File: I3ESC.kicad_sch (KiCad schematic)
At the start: 120 parts, among them J1 JST SR/SZ, J10 VIN_BARREL, J11 Barrel_Jack, J12 JST SR/SZ, J13 Conn_01x04, J2 Screw_Terminal_01x02, J3 Screw_Terminal_01x02, J4 Screw_Terminal_01x02, J5 Conn_01x06, J6 Wireless Coil, J7 VIN_TERMINAL, J8 Conn_01x06, J9 JST SR/SZ, SW2 boot-red, SW3 user1-white, U1 SY8113BADC, U10 USBLC6-2P6, U11 IP6826, U12 FD8288T (DRV8300), U2 FD8288T (DRV8300), U3 SPX3819M5-L-3-3, U4 STM32G474RETx, U5 Qwiic1, U6 USB_C_Receptacle, U8 ABM3B-8.000MHZ, U9 USB_C_Receptacle

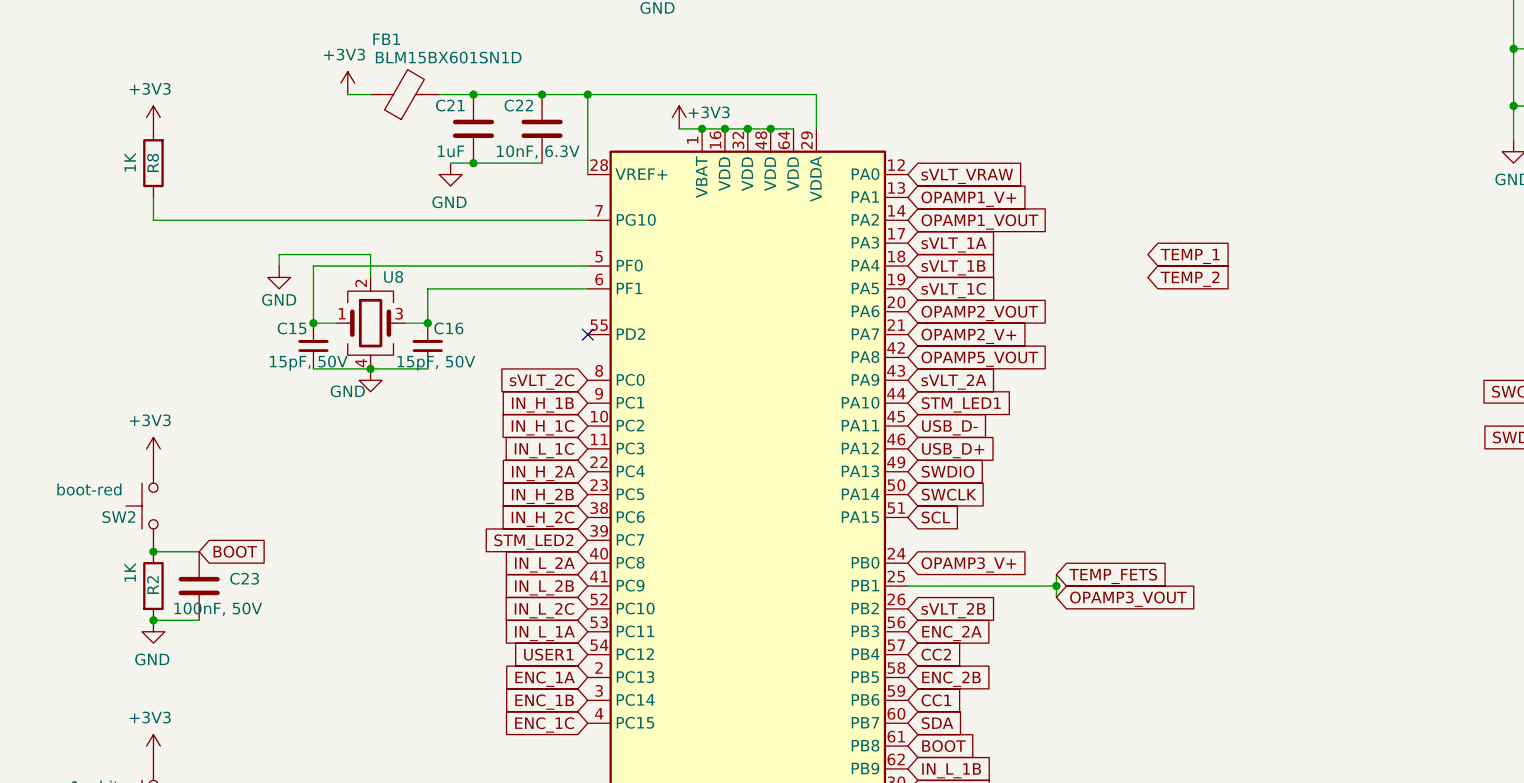
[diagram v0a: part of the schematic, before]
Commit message: majority of routing for V2 completed
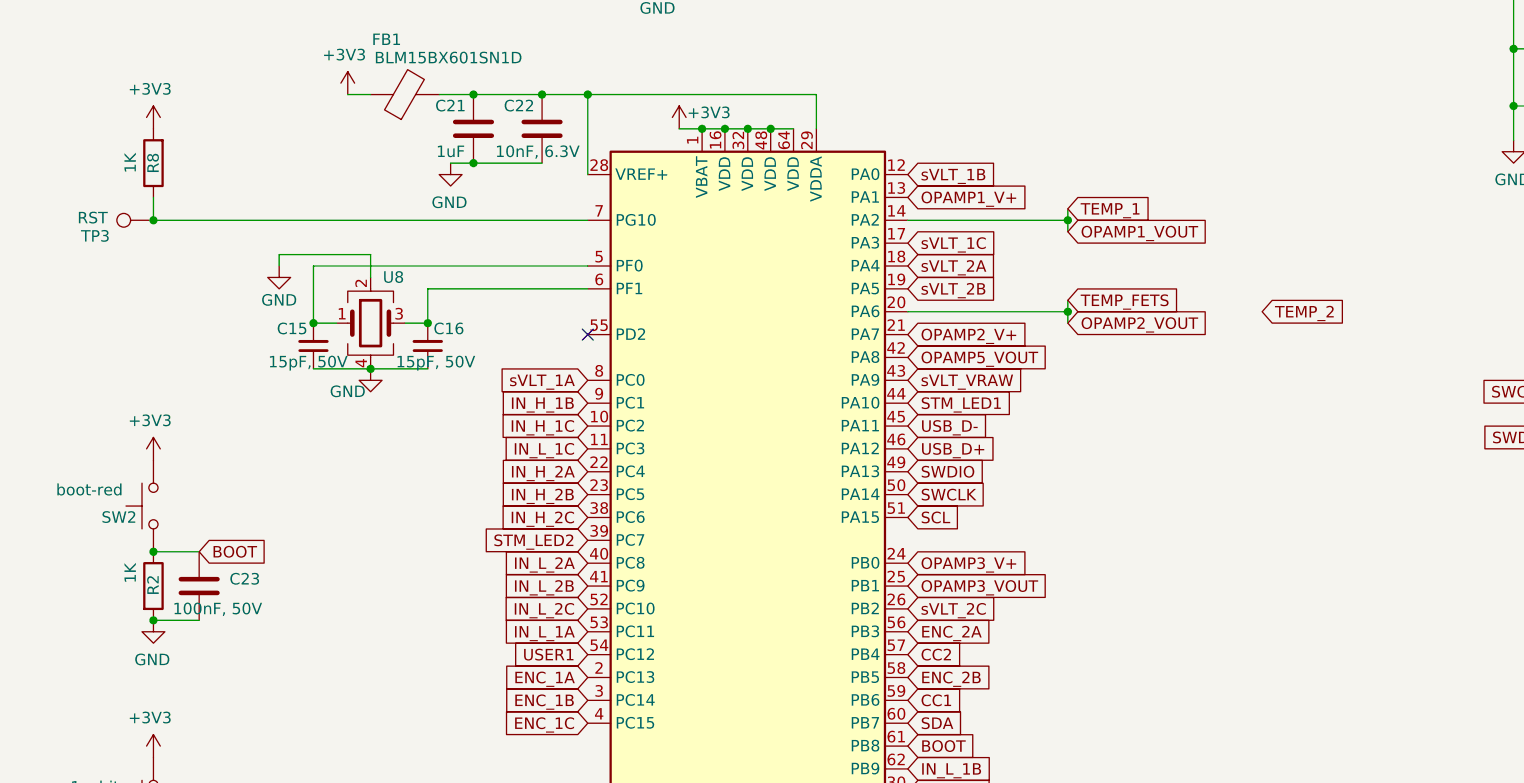
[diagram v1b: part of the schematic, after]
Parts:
- added TP3: RST, AlfredoFootprints:GE_TestPoint_Loop, symbol Connector:TestPoint
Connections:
- net TEMP_1 is gone; now on net OPAMP1_VOUT: J5.2 (Pin_2)
- net OPAMP2_VOUT: now also R40.2, R41.1
- net OPAMP3_VOUT: no longer R40.2, R41.1
- net sVLT_1A: now also U4.8 (PC0); no longer U4.17 (PA3)
- net sVLT_1B: now also U4.12 (PA0); no longer U4.18 (PA4)
- net sVLT_1C: now also U4.17 (PA3); no longer U4.19 (PA5)
- net sVLT_2A: now also U4.18 (PA4); no longer U4.43 (PA9)
- net sVLT_2B: now also U4.19 (PA5); no longer U4.26 (PB2)
- net sVLT_2C: now also U4.26 (PB2); no longer U4.8 (PC0)
- net sVLT_VRAW: now also U4.43 (PA9); no longer U4.12 (PA0)
- net at R8.1, U4.7 (PG10): now also TP3.1
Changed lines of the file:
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@@
 	)
 	(junction
+		(at -27.94 114.3)
+		(diameter 0)
+		(color 0 0 0 0)
+	)
+	(junction
 		(at 238.76 118.11)
 		(diameter 0)
@@
 	)
 	(junction
+		(at -129.54 114.3)
+		(diameter 0)
+		(color 0 0 0 0)
+	)
+	(junction
 		(at 184.15 133.35)
 		(diameter 0)
@@
 	)
 	(junction
-		(at -29.21 154.94)
-		(diameter 0)
-		(color 0 0 0 0)
-	)
-	(junction
 		(at 252.73 -59.69)
 		(diameter 0)
@@
 	)
 	(junction
+		(at -27.94 124.46)
+		(diameter 0)
+		(color 0 0 0 0)
+	)
+	(junction
 		(at -73.66 78.74)
 		(diameter 0)
@@
 	(wire
 		(pts
+			(xy -45.72 124.46) (xy -27.94 124.46)
+		)
+		(stroke
+			(width 0)
+			(type default)
+		)
+	)
+	(wire
+		(pts
 			(xy 274.32 -59.69) (xy 271.78 -59.69)
 		)
@@
 	(wire
 		(pts
+			(xy -45.72 114.3) (xy -27.94 114.3)
+		)
+		(stroke
+			(width 0)
+			(type default)
+		)
+	)
+	(wire
+		(pts
 			(xy -81.28 100.33) (xy -81.28 109.22)
 		)
@@
 	(wire
 		(pts
+			(xy -27.94 124.46) (xy -27.94 123.19)
+		)
+		(stroke
+			(width 0)
+			(type default)
+		)
+	)
+	(wire
+		(pts
 			(xy 87.63 -85.09) (xy 104.14 -85.09)
 		)
@@
 	(wire
 		(pts
-			(xy -29.21 153.67) (xy -29.21 154.94)
-		)
-		(stroke
-			(width 0)
-			(type default)
-		)
-	)
-	(wire
-		(pts
 			(xy 265.43 74.93) (xy 246.38 74.93)
 		)
@@
 	(wire
 		(pts
-			(xy -45.72 154.94) (xy -29.21 154.94)
-		)
-		(stroke
-			(width 0)
-			(type default)
-		)
-	)
-	(wire
-		(pts
 			(xy 153.67 67.31) (xy 160.02 67.31)
 		)
@@
 	(wire
 		(pts
+			(xy -27.94 114.3) (xy -27.94 115.57)
+		)
+		(stroke
+			(width 0)
+			(type default)
+		)
+	)
+	(wire
+		(pts
 			(xy -53.34 86.36) (xy -40.64 86.36)
 		)
@@
 	(wire
 		(pts
+			(xy -27.94 124.46) (xy -27.94 125.73)
+		)
+		(stroke
+			(width 0)
+			(type default)
+		)
+	)
+	(wire
+		(pts
 			(xy 295.91 -101.6) (xy 295.91 -96.52)
 		)
@@
 	(wire
 		(pts
-			(xy -29.21 154.94) (xy -29.21 156.21)
+			(xy 246.38 74.93) (xy 246.38 99.06)
 		)
 		(stroke
@@
 	(wire
 		(pts
-			(xy 246.38 74.93) (xy 246.38 99.06)
+			(xy -91.44 -68.58) (xy -72.39 -68.58)
 		)
 		(stroke
@@
 	(wire
 		(pts
-			(xy -91.44 -68.58) (xy -72.39 -68.58)
+			(xy 342.9 -101.6) (xy 339.09 -101.6)
 		)
 		(stroke
@@
 	(wire
 		(pts
-			(xy 342.9 -101.6) (xy 339.09 -101.6)
+			(xy 153.67 125.73) (xy 186.69 125.73)
 		)
 		(stroke
@@
 	(wire
 		(pts
-			(xy 153.67 125.73) (xy 186.69 125.73)
+			(xy -66.04 86.36) (xy -53.34 86.36)
 		)
 		(stroke
@@
 	(wire
 		(pts
-			(xy -66.04 86.36) (xy -53.34 86.36)
+			(xy 156.21 41.91) (xy 156.21 52.07)
 		)
 		(stroke
@@
 	(wire
 		(pts
-			(xy 156.21 41.91) (xy 156.21 52.07)
+			(xy 72.39 -60.96) (xy 72.39 -63.5)
 		)
 		(stroke
@@
 	(wire
 		(pts
-			(xy 72.39 -60.96) (xy 72.39 -63.5)
+			(xy -27.94 113.03) (xy -27.94 114.3)
 		)
 		(stroke
@@
 	(global_label "sVLT_2B"
 		(shape input)
-		(at -45.72 157.48 0)
+		(at -45.72 121.92 0)
 		(fields_autoplaced yes)
 		(effects
@@
 		)
 		(property "Intersheetrefs" "${INTERSHEET_REFS}"
-			(at -35.1753 157.48 0)
+			(at -35.1753 121.92 0)
 			(effects
 				(font
@@
 	(global_label "TEMP_1"
 		(shape input)
-		(at -19.05 118.11 0)
+		(at -27.94 113.03 0)
 		(fields_autoplaced yes)
 		(effects
@@
 		)
 		(property "Intersheetrefs" "${INTERSHEET_REFS}"
-			(at -9.0497 118.11 0)
+			(at -17.9397 113.03 0)
 			(effects
 				(font
@@
 	(global_label "sVLT_2A"
 		(shape input)
-		(at -45.72 132.08 0)
+		(at -45.72 119.38 0)
 		(fields_autoplaced yes)
 		(effects
@@
 		)
 		(property "Intersheetrefs" "${INTERSHEET_REFS}"
-			(at -35.3567 132.08 0)
+			(at -35.3567 119.38 0)
 			(effects
 				(font
@@
 	(global_label "OPAMP2_VOUT"
 		(shape input)
-		(at -45.72 124.46 0)
+		(at -27.94 125.73 0)
 		(fields_autoplaced yes)
 		(effects
@@
 		)
 		(property "Intersheetrefs" "${INTERSHEET_REFS}"
-			(at -29.43 124.46 0)
+			(at -11.65 125.73 0)
 			(effects
 				(font
@@
 	(global_label "sVLT_2C"
 		(shape input)
-		(at -81.28 132.08 180)
+		(at -45.72 157.48 0)
 		(fields_autoplaced yes)
 		(effects
@@
 				(size 1.27 1.27)
 			)
-			(justify right)
+			(justify left)
 		)
 		(property "Intersheetrefs" "${INTERSHEET_REFS}"
-			(at -91.8247 132.08 0)
+			(at -35.1753 157.48 0)
 			(effects
 				(font
 					(size 1.27 1.27)
 				)
-				(justify right)
+				(justify left)
 				(hide yes)
 			)
@@
 	(global_label "TEMP_FETS"
 		(shape input)
-		(at -29.21 153.67 0)
+		(at -27.94 123.19 0)
 		(fields_autoplaced yes)
 		(effects
@@
 		)
 		(property "Intersheetrefs" "${INTERSHEET_REFS}"
-			(at -16.5764 153.5906 0)
+			(at -15.3064 123.1106 0)
 			(effects
 				(font
@@
 	(global_label "TEMP_2"
 		(shape input)
-		(at -19.05 120.65 0)
+		(at -6.35 124.46 0)
 		(fields_autoplaced yes)
 		(effects
@@
 		)
 		(property "Intersheetrefs" "${INTERSHEET_REFS}"
-			(at -9.0497 120.65 0)
+			(at 3.6503 124.46 0)
 			(effects
 				(font
@@
 	(global_label "sVLT_1A"
 		(shape input)
-		(at -45.72 116.84 0)
+		(at -81.28 132.08 180)
 		(fields_autoplaced yes)
 		(effects
@@
 				(size 1.27 1.27)
 			)
-			(justify left)
+			(justify right)
 		)
 		(property "Intersheetrefs" "${INTERSHEET_REFS}"
-			(at -35.3567 116.84 0)
+			(at -91.6433 132.08 0)
 			(effects
 				(font
 					(size 1.27 1.27)
 				)
-				(justify left)
+				(justify right)
 				(hide yes)
 			)
@@
 	(global_label "sVLT_1B"
 		(shape input)
-		(at -45.72 119.38 0)
+		(at -45.72 109.22 0)
 		(fields_autoplaced yes)
 		(effects
@@
 		)
 		(property "Intersheetrefs" "${INTERSHEET_REFS}"
-			(at -35.1753 119.38 0)
+			(at -35.1753 109.22 0)
 			(effects
 				(font
@@
 	(global_label "sVLT_VRAW"
 		(shape input)
-		(at -45.72 109.22 0)
+		(at -45.72 132.08 0)
 		(fields_autoplaced yes)
 		(effects
@@
 		)
 		(property "Intersheetrefs" "${INTERSHEET_REFS}"
-			(at -32.7562 109.22 0)
+			(at -32.7562 132.08 0)
 			(effects
 				(font
@@
 	(global_label "OPAMP3_VOUT"
 		(shape input)
-		(at -29.21 156.21 0)
+		(at -45.72 154.94 0)
 		(fields_autoplaced yes)
 		(effects
@@
 		)
 		(property "Intersheetrefs" "${INTERSHEET_REFS}"
-			(at -12.92 156.21 0)
+			(at -29.43 154.94 0)
 			(effects
 				(font
@@
 	(global_label "sVLT_1C"
 		(shape input)
-		(at -45.72 121.92 0)
+		(at -45.72 116.84 0)
 		(fields_autoplaced yes)
 		(effects
@@
 		)
 		(property "Intersheetrefs" "${INTERSHEET_REFS}"
-			(at -35.1753 121.92 0)
+			(at -35.1753 116.84 0)
 			(effects
 				(font
@@
 	(global_label "OPAMP1_VOUT"
 		(shape input)
-		(at -45.72 114.3 0)
+		(at -27.94 115.57 0)
 		(fields_autoplaced yes)
 		(effects
@@
 		)
 		(property "Intersheetrefs" "${INTERSHEET_REFS}"
-			(at -29.43 114.3 0)
+			(at -11.65 115.57 0)
 			(effects
 				(font
@@
 					(unit 1)
 				)
+			)
+		)
+	)
+	(symbol
+		(lib_id "Connector:TestPoint")
+		(at -129.54 114.3 90)
+		(unit 1)
+		(exclude_from_sim no)
+		(in_bom yes)
+		(on_board yes)
+		(dnp no)
+		(property "Reference" "TP3"
+			(at -134.366 116.078 90)
+			(effects
+				(font
+					(size 1.27 1.27)
+				)
+				(justify left)
+			)
+		)
+		(property "Value" "RST"
+			(at -134.62 114.046 90)
+			(effects
+				(font
+					(size 1.27 1.27)
+				)
+				(justify left)
+			)
+		)
+		(property "Footprint" "AlfredoFootprints:GE_TestPoint_Loop"
+			(at -129.54 109.22 0)
+			(effects
+				(font
+					(size 1.27 1.27)
+				)
+				(hide yes)
+			)
+		)
+		(property "Datasheet" "~"
+			(at -129.54 109.22 0)
+			(effects
+				(font
+					(size 1.27 1.27)
+				)
+				(hide yes)
+			)
+		)
+		(property "Description" ""
+			(at -129.54 114.3 0)
+			(effects
+				(font
+					(size 1.27 1.27)
+				)
+				(hide yes)
+			)
+		)
+		(property "LCSC" "~"
+			(at -129.54 114.3 0)
+			(effects
+				(font
+					(size 1.27 1.27)
+				)
+				(hide yes)
+			)
+		)
+		(pin "1"
+		)
+		(instances
+			(project "I3ESC"
+				(path "/718f3b0f-9bd0-4d7b-8c07-e00d61b06ce3"
+					(reference "TP3")
+					(unit 1)
+				)

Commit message: push before schematic cleanup
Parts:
- removed TP5: TP_CC2, AlfredoFootprints:GE_TestPoint_Loop, symbol Connector:TestPoint
- removed TP6: TP_CC1, AlfredoFootprints:GE_TestPoint_Loop, symbol Connector:TestPoint
- C27, C28, C32: footprint Capacitor_SMD:C_0402_1005Metric -> Capacitor_SMD:C_0603_1608Metric; LCSC C307331 -> C14663
- C30, C31: footprint Capacitor_SMD:C_0402_1005Metric -> Capacitor_SMD:C_0603_1608Metric; LCSC C696852 -> C1596
- D10, D84: LCSC (none) -> C965804
- D7: value LED_RED -> LED_YELLOW; LCSC (none) -> C72038
- D83: LCSC (none) -> C965807
- D9: value LED_Red -> LED_YELLOW; LCSC (none) -> C72038
- JP2: value VCC-bypass -> VCC_bypass
- R20, R26, R27: footprint Resistor_SMD:R_0402_1005Metric -> Resistor_SMD:R_0603_1608Metric; LCSC C25741 -> C25803
- R28, R29: footprint Resistor_SMD:R_0402_1005Metric -> Resistor_SMD:R_0603_1608Metric; LCSC C11702 -> C21190
- R34: footprint Resistor_SMD:R_0402_1005Metric -> Resistor_SMD:R_0603_1608Metric; LCSC C25744 -> C25804
- R35: footprint Resistor_SMD:R_0402_1005Metric -> Resistor_SMD:R_0603_1608Metric; LCSC C25779 -> C4216
- R9: footprint Resistor_SMD:R_0402_1005Metric -> Resistor_SMD:R_0603_1608Metric; LCSC C25890 -> C22978
- U4: LCSC (none) -> C521608
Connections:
- net TEMP_2 is gone; now on net OPAMP5_VOUT: J8.2 (Pin_2)
- net IE-FETS-2B/VOUT: now also J11.2; no longer J11.1
- net IE-FETS-2C/VOUT: now also J11.1; no longer J11.2
- net Qi_CC1: now also U11.8 (CC1)
- net Qi_CC2: now also U11.9 (CC2)
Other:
- added sheet Untitled Sheet (untitled.kicad_sch)
- note added: "long term: - max VIN is 18V from buck converter (upgrade?) - switch to smaller pkg drv SIG TODO: - better test probes POWER TODO: -pick new barrel jack? done: - improve SWD interface? (or is 4 pin jst good?) - change G432 to G474 - Boot button is actually rst (fix this) - add boot button for DFU - no way to measure battery current sns with barrel out? - mode buttons with indicator - Bulk up RPP f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"
- note removed: "long term: - max VIN is 18V from buck converter (upgrade?) - switch to smaller pkg drv SIG TODO: - better test probes - attach TEMP1 and TEMP2 to VOUT pins - fix wireless charger - change wireless chips to 0603 POWER TODO: - find power diode for D8 -pick new barrel jack? done: - improve SWD interface? (or is 4 pin jst good?) - change G432 to G474 - Boot button is actually rst (fix this) - add boo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"
